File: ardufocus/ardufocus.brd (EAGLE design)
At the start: 50 x 63 mm, 18 parts, among them J5 POWER_JACK, M1 ARDUINO-NANO-3.0, X2 JST-XH-04-PIN-LONG-PAD, X3 JST-XH-04-PIN-LONG-PAD, X4 JST-XH-04-PIN-LONG-PAD, X5 JST-XH-04-PIN-LONG-PAD, X6 JST-XH-02-PIN-LONG-PAD

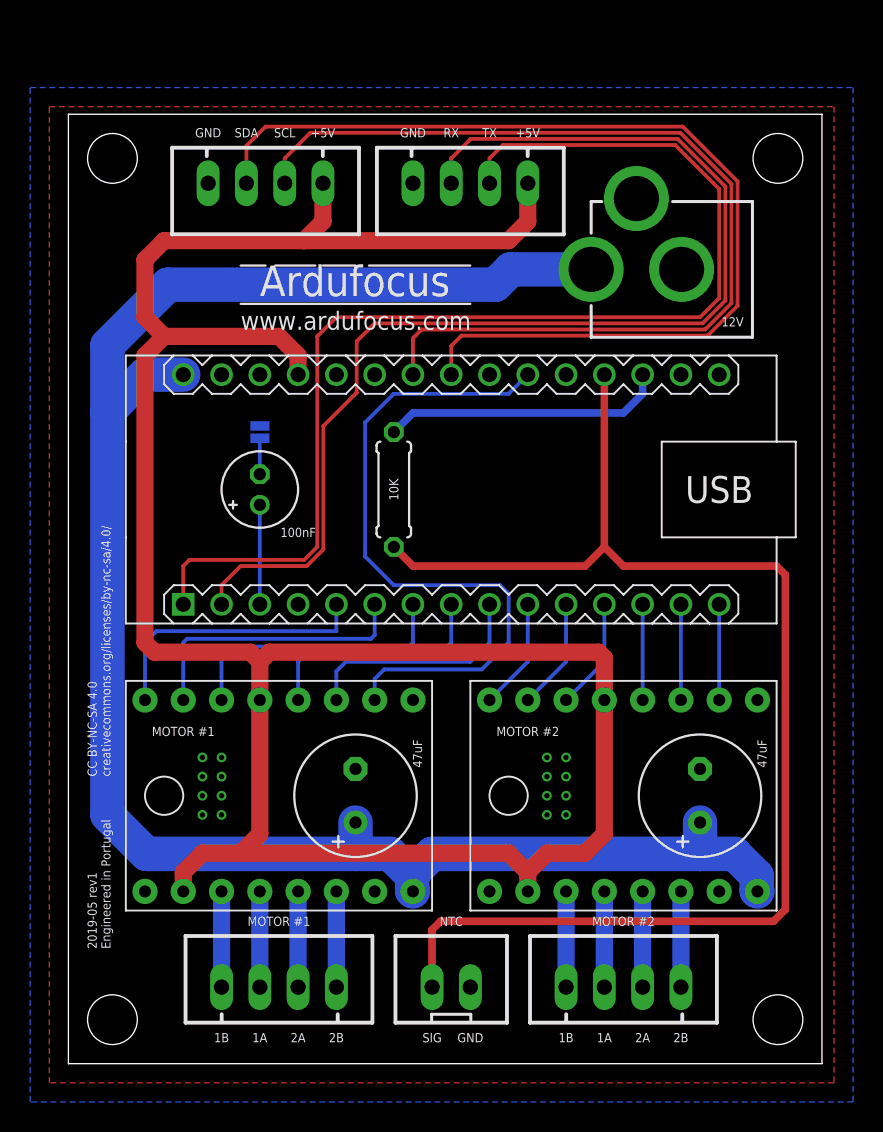
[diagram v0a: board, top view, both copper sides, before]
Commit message: New PCB layout
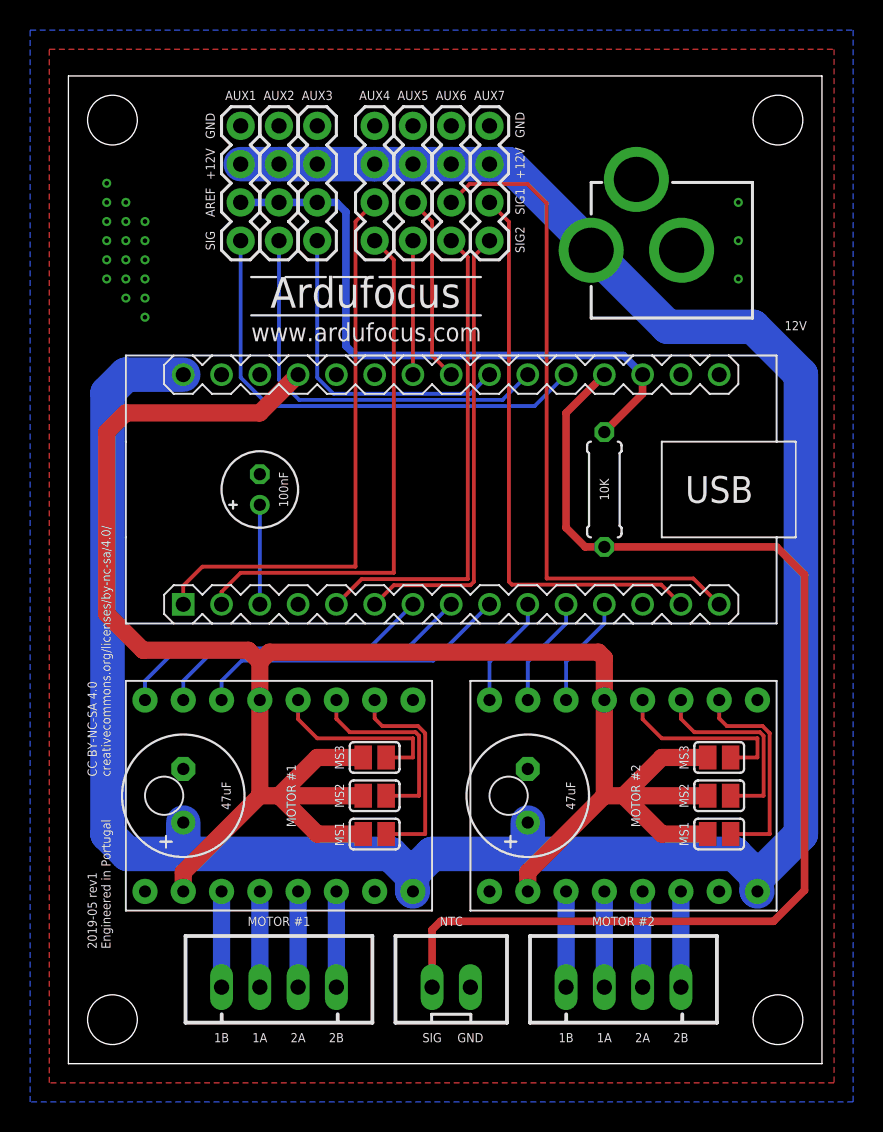
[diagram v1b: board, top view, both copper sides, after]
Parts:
- removed J5: POWER_JACK, SparkFun-Connectors:POWER_JACK_PTH
- removed PGRM: JUMPER-SMT_2_NO_SILK, SparkFun-Jumpers:SMT-JUMPER_2_NO_SILK
- removed X4, X5: JST-XH-04-PIN-LONG-PAD, jst-xh:JST-XH-04-PACKAGE-LONG-PAD
- added 01MS2, O1MS1, O1MS3, O2MS1, O2MS2, O2MS3: (no value), jumper:SJ
- added AUX1, AUX2, AUX3: Analog, SparkFun-Connectors:1X04
- added AUX4: HW Serial, SparkFun-Connectors:1X04
- added AUX5: I2C, SparkFun-Connectors:1X04
- added AUX6, AUX7: (no value), SparkFun-Connectors:1X04
- added J1: POWER_JACK, SparkFun-Connectors:POWER_JACK_PTH
- moved R1 14.0 mm to (35.6, 38.1)
- moved C2 11.4 mm to (7.62, 17.8)
- moved C3 11.4 mm to (30.5, 17.8)
- moved U$1 2.54 mm to (2.92, 62.6)
- moved U$3 2.54 mm to (47.1, 62.6)
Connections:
- removed net N$2: C1.-, PGRM.1
- new net O1MS1: O1MS1.2, OUT1.MS1
- new net O1MS2: 01MS2.2, OUT1.MS2
- new net O1MS3: O1MS3.2, OUT1.MS3
- new net O2MS1: O2MS1.2, OUT2.MS1
- new net O2MS2: O2MS2.2, OUT2.MS2
- new net O2MS3: O2MS3.2, OUT2.MS3
- net +12V: now also AUX1.2, AUX2.2, AUX3.2, AUX4.2, AUX5.2, AUX6.2, AUX7.2, J1.PWR; no longer J5.PWR
- net +5V: now also 01MS2.1, O1MS1.1, O1MS3.1, O2MS1.1, O2MS2.1, O2MS3.1; no longer X4.1, X5.1
- net A1: now also AUX1.4
- net A2: now also AUX2.4; no longer OUT1.MS1
- net A3: now also AUX3.4
- net AREF: now also AUX1.3, AUX2.3, AUX3.3
- net D10: no longer OUT2.MS3
- net D11: now also AUX7.3; no longer OUT2.MS2
- net D12: now also AUX6.3; no longer OUT2.MS1
- net D2: now also AUX6.4; no longer OUT1.DIR
- net D3: now also AUX7.4; no longer OUT1.STEP
- net D4: now also OUT1.DIR; no longer OUT1.SLEEP
- net D5: now also OUT1.STEP; no longer OUT1.MS3
- net D6: now also OUT1.SLEEP; no longer OUT1.MS2
- net GND: now also AUX1.1, AUX2.1, AUX3.1, AUX4.1, AUX5.1, AUX6.1, AUX7.1, C1.-, J1.GND; no longer J5.GND, PGRM.2, X4.4, X5.4
- net RX: now also AUX4.4; no longer X4.3
- net SCL: now also AUX5.4; no longer X5.2
- net SDA: now also AUX5.3; no longer X5.3
- net TX: now also AUX4.3; no longer X4.2
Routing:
- net SCL: track 65.8 -> 8.89 mm
- net SDA: track 67.4 -> 12.5 mm
- net RX: track 78.6 -> 35.3 mm
- net TX: track 79.4 -> 37.9 mm
- net +12V: track 123.7 -> 164.2 mm
- net D12: track 6.35 -> 44.4 mm
- net A1: track 0.00 -> 32.3 mm
- net D11: track 6.35 -> 37.7 mm
- net +5V: track 159.4 -> 136.3 mm
- net AREF: track 18.8 -> 41.5 mm
- net A3: track 0.00 -> 21.5 mm
- net A2: track 46.1 -> 27.0 mm
- net O2MS1: track 0.00 -> 14.3 mm
- net O1MS1: track 0.00 -> 14.3 mm
- net D2: track 18.6 -> 32.3 mm
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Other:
- board size 50 x 63 mm -> 50 x 65.5 mm
- board text added: "+12V"
- board text added: "AREF"
- board text added: "AUX1"
- board text added: "AUX2"
- board text added: "AUX3"
- board text added: "AUX4"
- board text added: "AUX5"
- board text added: "AUX6"
- board text added: "AUX7"
- board text added: "MS1"
- board text added: "MS2"
- board text added: "MS3"
- board text added: "SIG1"
- board text added: "SIG2"
- board text removed: "+5V"
- board text removed: "RX"
- board text removed: "SCL"
- board text removed: "SDA"
- board text removed: "TX"

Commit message: Revert "New PCB layout"
This reverts commit abb039d9954214917f7d505cd5213ebb6519a360.
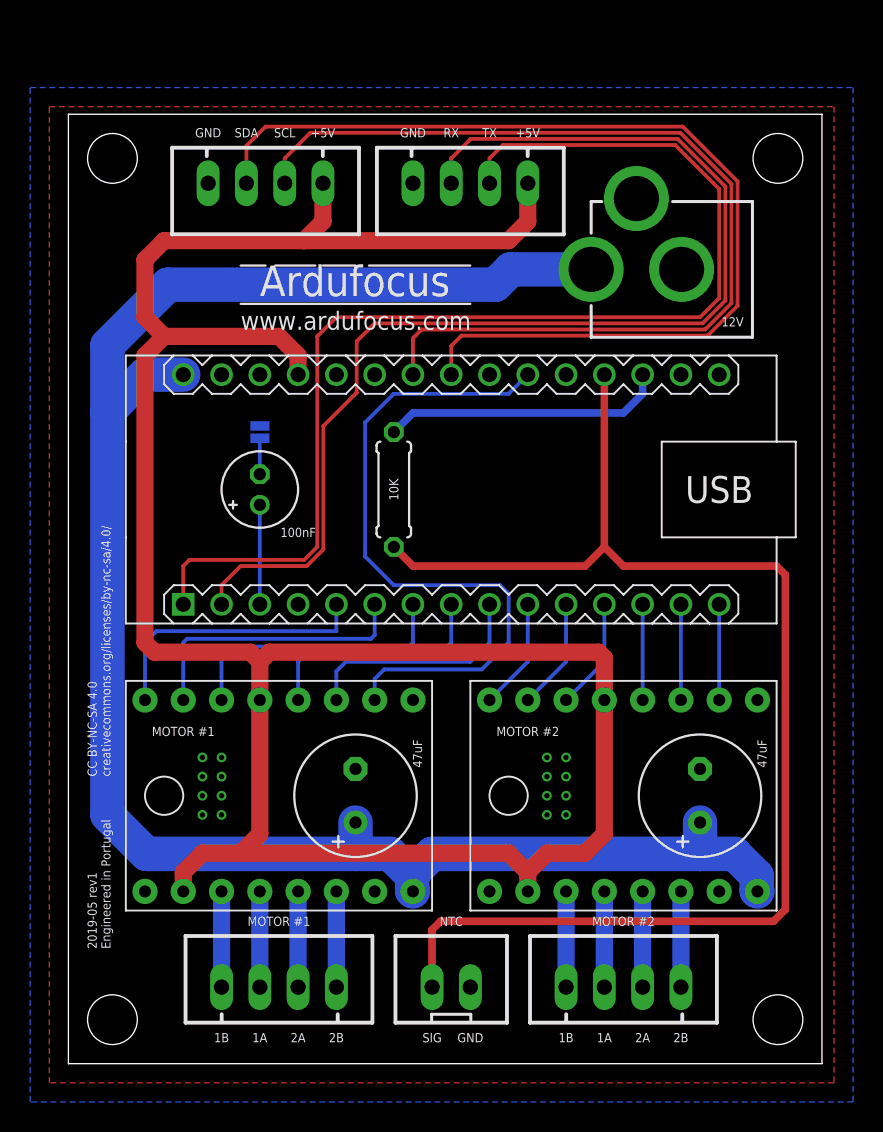
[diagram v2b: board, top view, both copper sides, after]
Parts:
- removed 01MS2, O1MS1, O1MS3, O2MS1, O2MS2, O2MS3: (no value), jumper:SJ
- removed AUX1, AUX2, AUX3: Analog, SparkFun-Connectors:1X04
- removed AUX4: HW Serial, SparkFun-Connectors:1X04
- removed AUX5: I2C, SparkFun-Connectors:1X04
- removed AUX6, AUX7: (no value), SparkFun-Connectors:1X04
- removed J1: POWER_JACK, SparkFun-Connectors:POWER_JACK_PTH
- added J5: POWER_JACK, SparkFun-Connectors:POWER_JACK_PTH
- added PGRM: JUMPER-SMT_2_NO_SILK, SparkFun-Jumpers:SMT-JUMPER_2_NO_SILK
- added X4, X5: JST-XH-04-PIN-LONG-PAD, jst-xh:JST-XH-04-PACKAGE-LONG-PAD
- moved R1 14.0 mm to (21.6, 38.1)
- moved C2 11.4 mm to (19.1, 17.8)
- moved C3 11.4 mm to (41.9, 17.8)
- moved U$1 2.54 mm to (2.92, 60.1)
- moved U$3 2.54 mm to (47.1, 60.1)
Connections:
- removed net O1MS1: O1MS1.2, OUT1.MS1
- removed net O1MS2: 01MS2.2, OUT1.MS2
- removed net O1MS3: O1MS3.2, OUT1.MS3
- removed net O2MS1: O2MS1.2, OUT2.MS1
- removed net O2MS2: O2MS2.2, OUT2.MS2
- removed net O2MS3: O2MS3.2, OUT2.MS3
- new net N$2: C1.-, PGRM.1
- net +12V: now also J5.PWR; no longer AUX1.2, AUX2.2, AUX3.2, AUX4.2, AUX5.2, AUX6.2, AUX7.2, J1.PWR
- net +5V: now also X4.1, X5.1; no longer 01MS2.1, O1MS1.1, O1MS3.1, O2MS1.1, O2MS2.1, O2MS3.1
- net A1: no longer AUX1.4
- net A2: now also OUT1.MS1; no longer AUX2.4
- net A3: no longer AUX3.4
- net AREF: no longer AUX1.3, AUX2.3, AUX3.3
- net D10: now also OUT2.MS3
- net D11: now also OUT2.MS2; no longer AUX7.3
- net D12: now also OUT2.MS1; no longer AUX6.3
- net D2: now also OUT1.DIR; no longer AUX6.4
- net D3: now also OUT1.STEP; no longer AUX7.4
- net D4: now also OUT1.SLEEP; no longer OUT1.DIR
- net D5: now also OUT1.MS3; no longer OUT1.STEP
- net D6: now also OUT1.MS2; no longer OUT1.SLEEP
- net GND: now also J5.GND, PGRM.2, X4.4, X5.4; no longer AUX1.1, AUX2.1, AUX3.1, AUX4.1, AUX5.1, AUX6.1, AUX7.1, C1.-, J1.GND
- net RX: now also X4.3; no longer AUX4.4
- net SCL: now also X5.2; no longer AUX5.4
- net SDA: now also X5.3; no longer AUX5.3
- net TX: now also X4.2; no longer AUX4.3
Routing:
- net SCL: track 8.89 -> 65.8 mm
- net SDA: track 12.5 -> 67.4 mm
- net RX: track 35.3 -> 78.6 mm
- net TX: track 37.9 -> 79.4 mm
- net +12V: track 164.2 -> 123.7 mm
- net D12: track 44.4 -> 6.35 mm
- net A1: track 32.3 -> 0.00 mm
- net D11: track 37.7 -> 6.35 mm
- net +5V: track 136.3 -> 159.4 mm
- net AREF: track 41.5 -> 18.8 mm
- net A3: track 21.5 -> 0.00 mm
- net A2: track 27.0 -> 46.1 mm
- net O2MS1: track 14.3 -> 0.00 mm
- net O1MS1: track 14.3 -> 0.00 mm
- net D2: track 32.3 -> 18.6 mm
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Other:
- board size 50 x 65.5 mm -> 50 x 63 mm
- board text added: "+5V"
- board text added: "RX"
- board text added: "SCL"
- board text added: "SDA"
- board text added: "TX"
- board text removed: "+12V"
- board text removed: "AREF"
- board text removed: "AUX1"
- board text removed: "AUX2"
- board text removed: "AUX3"
- board text removed: "AUX4"
- board text removed: "AUX5"
- board text removed: "AUX6"
- board text removed: "AUX7"
- board text removed: "MS1"
- board text removed: "MS2"
- board text removed: "MS3"
- board text removed: "SIG1"
- board text removed: "SIG2"
